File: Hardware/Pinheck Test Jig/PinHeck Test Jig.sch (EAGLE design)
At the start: 314 parts, among them U1 P8X32A-Q44, U10 BSO080P03NS3E G, U11 BSO080P03NS3E G, U12 MF-DSC-SOT233-MMBT3904, U13 MF-DSC-SOT233-MMBT3904, U14 CD74HC595M96, U15 CD74HC595M96, U16 CD74HC165M96, U17 CD74HC165M96, U18 CD74HC165M96, U19 CD74HC165M96, U2 CAT24C512WI-GT3, U20 CD74HC165M96, U21 CD74HC165M96, U22 CD74HC165M96, U23 CD74HC165M96, U24 CD74HC165M96, U26 CD74HC165M96, U27 CD74HC165M96, U28 CD74HC165M96, U29 CD74HC165M96, U3 FT230XS, U30 CD74HC165M96, U4 IP4234CZ6, U5 NCP1117DT33G, U6 NCP1117DT50G, U7 INA139NA/3K, U8 INA139NA/3K, U9 MAX11613EUA+, X1 ABMM-6.000MHZ-B2-T

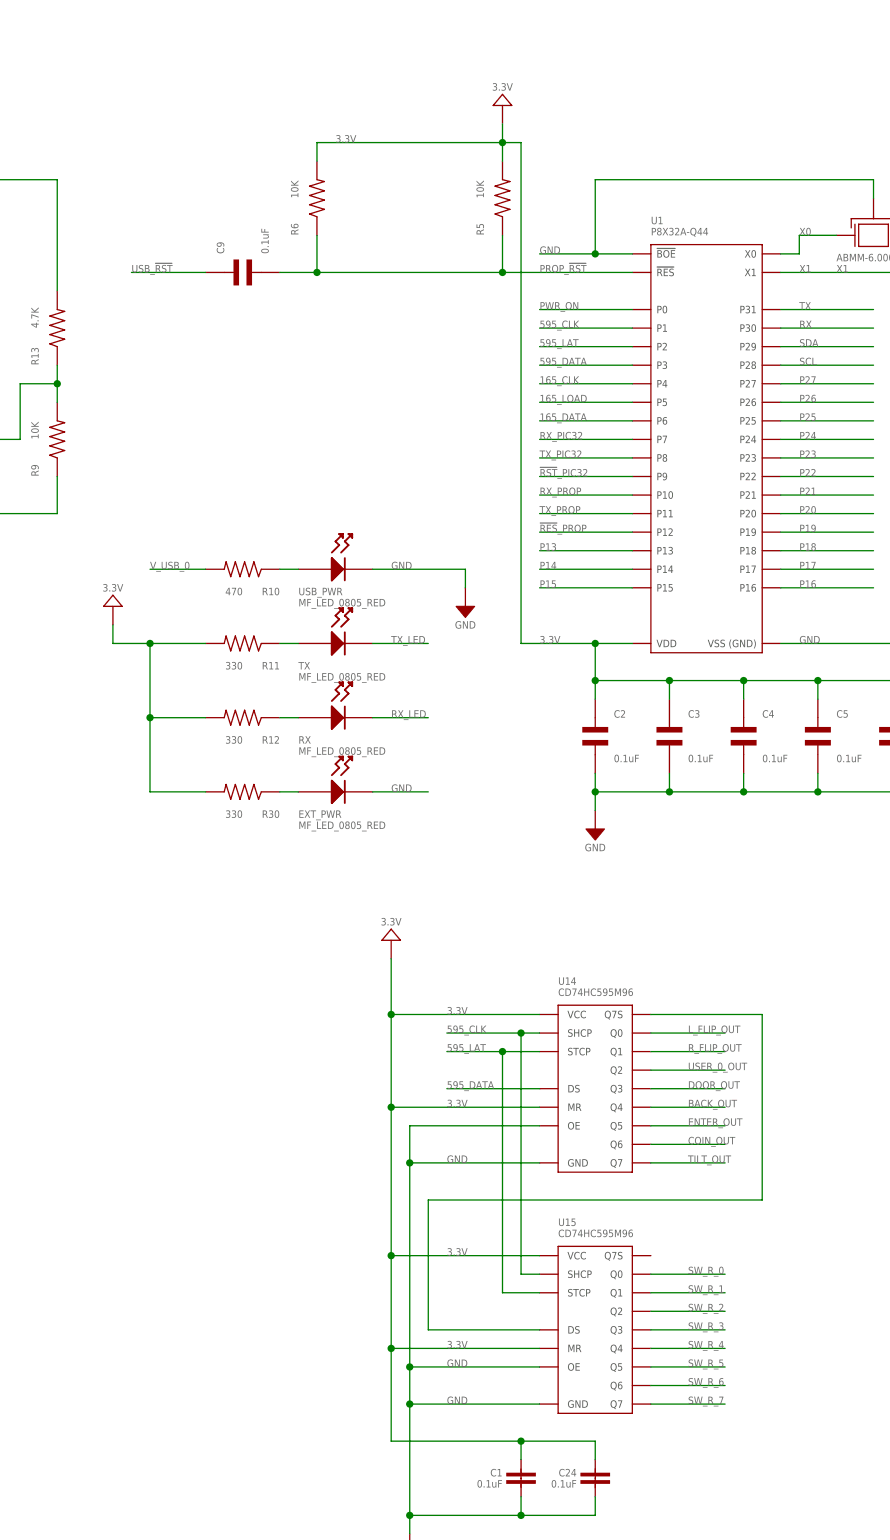
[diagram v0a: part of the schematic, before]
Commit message: Still routing!
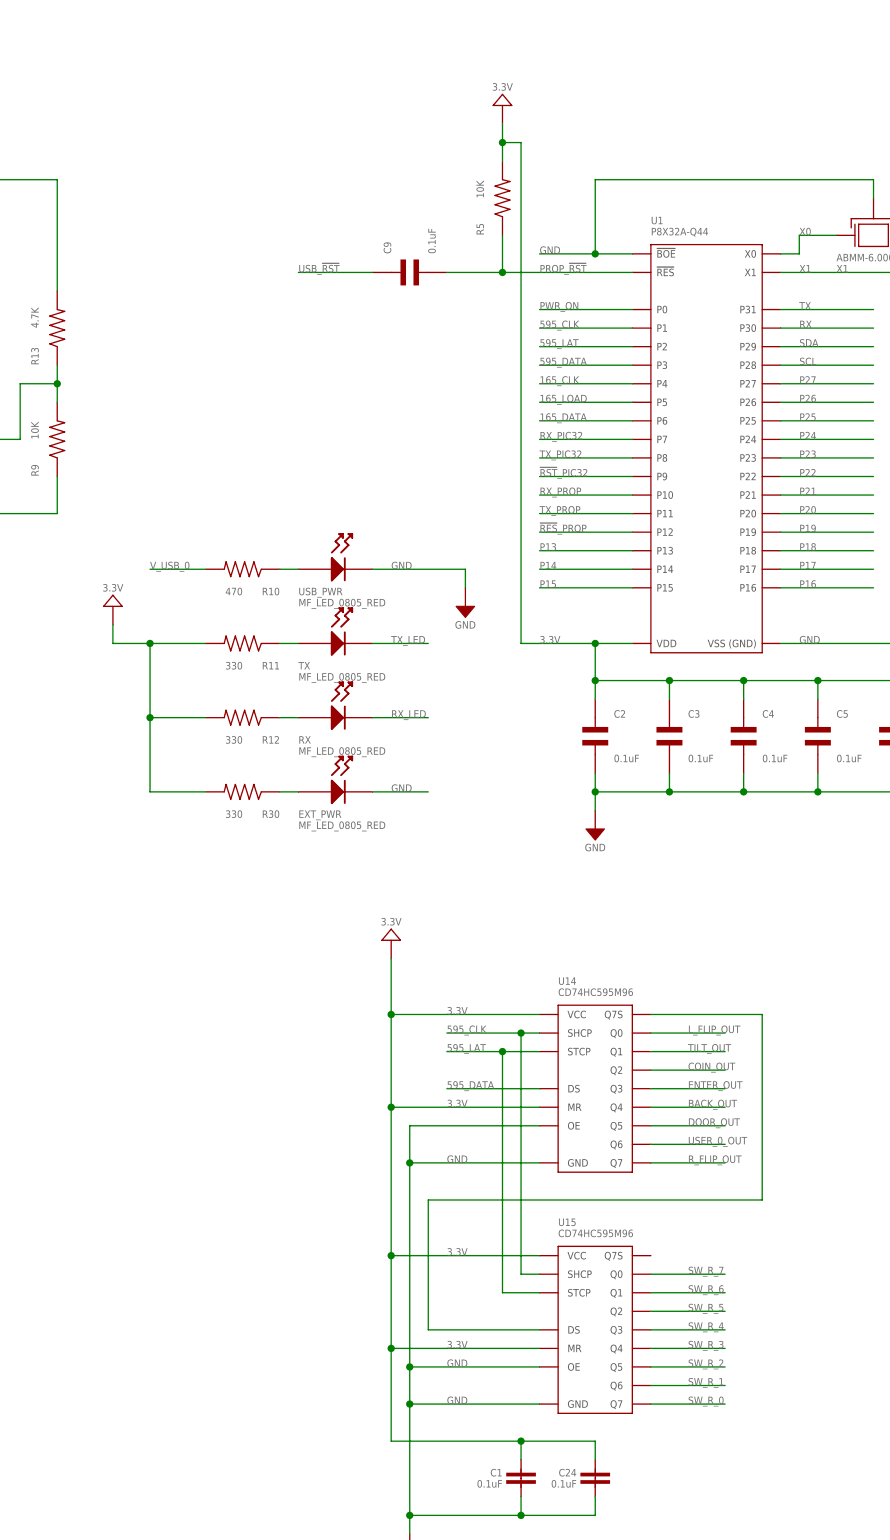
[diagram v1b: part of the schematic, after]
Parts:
- removed R6: 10K, MF_Passives:RESISTOR_0603
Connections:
- net 3.3V: no longer R6.P$2
- net COIN_OUT: now also U14.Q2; no longer U14.Q6
- net DOOR_OUT: now also U14.Q5; no longer U14.Q3
- net ENTER_OUT: now also U14.Q3; no longer U14.Q5
- net PROP_!RST: no longer R6.P$1
- net R_FLIP_OUT: now also U14.Q7; no longer U14.Q1
- net SW_R_0: now also U15.Q7; no longer U15.Q0
- net SW_R_1: now also U15.Q6; no longer U15.Q1
- net SW_R_2: now also U15.Q5; no longer U15.Q2
- net SW_R_3: now also U15.Q4; no longer U15.Q3
- net SW_R_4: now also U15.Q3; no longer U15.Q4
- net SW_R_5: now also U15.Q2; no longer U15.Q5
- net SW_R_6: now also U15.Q1; no longer U15.Q6
- net SW_R_7: now also U15.Q0; no longer U15.Q7
- net TILT_OUT: now also U14.Q1; no longer U14.Q7
- net USER_0_OUT: now also U14.Q6; no longer U14.Q2
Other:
- moved on the sheet: C9
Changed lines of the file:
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@@
 <?xml version="1.0" encoding="utf-8"?>
 <!DOCTYPE eagle SYSTEM "eagle.dtd">
-<eagle version="6.6.0">
+<eagle version="6.5.0">
 <drawing>
 <settings>
@@
 <part name="C6" library="MF_Passives" deviceset="CAPACITOR_NP" device="_0603" value="0.1uF"/>
 <part name="R5" library="MF_Passives" deviceset="RESISTOR" device="_0603" value="10K"/>
-<part name="R6" library="MF_Passives" deviceset="RESISTOR" device="_0603" value="10K"/>
 <part name="U3" library="MF_IC_Digital" deviceset="FT230X" device="S"/>
 <part name="U4" library="PP_Passives" deviceset="IP4234CZ6" device="" value="IP4234CZ6"/>
@@
 <instance part="C6" gate="G$1" x="190.5" y="172.72"/>
 <instance part="R5" gate="G$1" x="81.28" y="175.26" rot="R90"/>
-<instance part="R6" gate="G$1" x="55.88" y="175.26" rot="R90"/>
 <instance part="U3" gate="G$1" x="-17.78" y="165.1"/>
 <instance part="U4" gate="G$1" x="-91.44" y="152.4" rot="R90"/>
@@
 <instance part="J1" gate="G$1" x="-129.54" y="160.02"/>
 <instance part="L1" gate="G$1" x="-111.76" y="132.08"/>
-<instance part="C9" gate="G$1" x="45.72" y="165.1" rot="R90"/>
+<instance part="C9" gate="G$1" x="68.58" y="165.1" rot="R90"/>
 <instance part="C10" gate="G$1" x="-30.48" y="144.78"/>
 <instance part="C11" gate="G$1" x="-45.72" y="144.78"/>
@@
 <pinref part="R5" gate="G$1" pin="P$2"/>
 <wire x1="81.28" y1="180.34" x2="81.28" y2="182.88" width="0.1524" layer="91"/>
-<wire x1="81.28" y1="182.88" x2="55.88" y2="182.88" width="0.1524" layer="91"/>
-<pinref part="R6" gate="G$1" pin="P$2"/>
-<wire x1="55.88" y1="182.88" x2="55.88" y2="180.34" width="0.1524" layer="91"/>
-<label x="58.42" y="182.88" size="1.016" layer="95" font="vector"/>
 <pinref part="U$12" gate="G$1" pin="P$1"/>
 <wire x1="81.28" y1="182.88" x2="81.28" y2="185.42" width="0.1524" layer="91"/>
@@
 </segment>
 <segment>
-<pinref part="U15" gate="G$1" pin="Q6"/>
-<wire x1="111.76" y1="12.7" x2="101.6" y2="12.7" width="0.1524" layer="91"/>
-<label x="106.68" y="12.7" size="1.016" layer="95" font="vector"/>
+<pinref part="U15" gate="G$1" pin="Q1"/>
+<wire x1="101.6" y1="25.4" x2="111.76" y2="25.4" width="0.1524" layer="91"/>
+<label x="106.68" y="25.4" size="1.016" layer="95" font="vector"/>
 </segment>
 </net>
@@
 </segment>
 <segment>
-<pinref part="U15" gate="G$1" pin="Q5"/>
-<wire x1="101.6" y1="15.24" x2="111.76" y2="15.24" width="0.1524" layer="91"/>
-<label x="106.68" y="15.24" size="1.016" layer="95" font="vector"/>
+<pinref part="U15" gate="G$1" pin="Q2"/>
+<wire x1="111.76" y1="22.86" x2="101.6" y2="22.86" width="0.1524" layer="91"/>
+<label x="106.68" y="22.86" size="1.016" layer="95" font="vector"/>
 </segment>
 </net>
@@
 </segment>
 <segment>
-<pinref part="U15" gate="G$1" pin="Q4"/>
-<wire x1="111.76" y1="17.78" x2="101.6" y2="17.78" width="0.1524" layer="91"/>
-<label x="106.68" y="17.78" size="1.016" layer="95" font="vector"/>
+<pinref part="U15" gate="G$1" pin="Q3"/>
+<wire x1="101.6" y1="20.32" x2="111.76" y2="20.32" width="0.1524" layer="91"/>
+<label x="106.68" y="20.32" size="1.016" layer="95" font="vector"/>
 </segment>
 </net>
@@
 </segment>
 <segment>
-<pinref part="U15" gate="G$1" pin="Q3"/>
-<wire x1="101.6" y1="20.32" x2="111.76" y2="20.32" width="0.1524" layer="91"/>
-<label x="106.68" y="20.32" size="1.016" layer="95" font="vector"/>
+<pinref part="U15" gate="G$1" pin="Q4"/>
+<wire x1="111.76" y1="17.78" x2="101.6" y2="17.78" width="0.1524" layer="91"/>
+<label x="106.68" y="17.78" size="1.016" layer="95" font="vector"/>
 </segment>
 </net>
@@
 </segment>
 <segment>
-<pinref part="U15" gate="G$1" pin="Q1"/>
-<wire x1="101.6" y1="25.4" x2="111.76" y2="25.4" width="0.1524" layer="91"/>
-<label x="106.68" y="25.4" size="1.016" layer="95" font="vector"/>
+<pinref part="U15" gate="G$1" pin="Q6"/>
+<wire x1="111.76" y1="12.7" x2="101.6" y2="12.7" width="0.1524" layer="91"/>
+<label x="106.68" y="12.7" size="1.016" layer="95" font="vector"/>
 </segment>
 </net>
@@
 </segment>
 <segment>
-<pinref part="U15" gate="G$1" pin="Q0"/>
-<wire x1="101.6" y1="27.94" x2="111.76" y2="27.94" width="0.1524" layer="91"/>
-<label x="106.68" y="27.94" size="1.016" layer="95" font="vector"/>
+<pinref part="U15" gate="G$1" pin="Q7"/>
+<wire x1="101.6" y1="10.16" x2="111.76" y2="10.16" width="0.1524" layer="91"/>
+<label x="106.68" y="10.16" size="1.016" layer="95" font="vector"/>
 </segment>
 </net>
@@
 </segment>
 <segment>
-<pinref part="U15" gate="G$1" pin="Q7"/>
-<wire x1="101.6" y1="10.16" x2="111.76" y2="10.16" width="0.1524" layer="91"/>
-<label x="106.68" y="10.16" size="1.016" layer="95" font="vector"/>
+<pinref part="U15" gate="G$1" pin="Q0"/>
+<wire x1="101.6" y1="27.94" x2="111.76" y2="27.94" width="0.1524" layer="91"/>
+<label x="106.68" y="27.94" size="1.016" layer="95" font="vector"/>
 </segment>
 </net>
@@
 </segment>
 <segment>
-<pinref part="U15" gate="G$1" pin="Q2"/>
-<wire x1="111.76" y1="22.86" x2="101.6" y2="22.86" width="0.1524" layer="91"/>
-<label x="106.68" y="22.86" size="1.016" layer="95" font="vector"/>
+<pinref part="U15" gate="G$1" pin="Q5"/>
+<wire x1="101.6" y1="15.24" x2="111.76" y2="15.24" width="0.1524" layer="91"/>
+<label x="106.68" y="15.24" size="1.016" layer="95" font="vector"/>
 </segment>
 </net>
@@
 </segment>
 <segment>
-<pinref part="U14" gate="G$1" pin="Q7"/>
-<wire x1="101.6" y1="43.18" x2="111.76" y2="43.18" width="0.1524" layer="91"/>
-<label x="106.68" y="43.18" size="1.016" layer="95" font="vector"/>
+<pinref part="U14" gate="G$1" pin="Q1"/>
+<wire x1="101.6" y1="58.42" x2="111.76" y2="58.42" width="0.1524" layer="91"/>
+<label x="106.68" y="58.42" size="1.016" layer="95" font="vector"/>
 </segment>
 </net>
@@
 </segment>
 <segment>
-<pinref part="U14" gate="G$1" pin="Q6"/>
-<wire x1="111.76" y1="45.72" x2="101.6" y2="45.72" width="0.1524" layer="91"/>
-<label x="106.68" y="45.72" size="1.016" layer="95" font="vector"/>
+<pinref part="U14" gate="G$1" pin="Q2"/>
+<wire x1="111.76" y1="55.88" x2="101.6" y2="55.88" width="0.1524" layer="91"/>
+<label x="106.68" y="55.88" size="1.016" layer="95" font="vector"/>
 </segment>
 </net>
@@
 </segment>
 <segment>
-<pinref part="U14" gate="G$1" pin="Q5"/>
-<wire x1="101.6" y1="48.26" x2="111.76" y2="48.26" width="0.1524" layer="91"/>
-<label x="106.68" y="48.26" size="1.016" layer="95" font="vector"/>
+<pinref part="U14" gate="G$1" pin="Q3"/>
+<wire x1="101.6" y1="53.34" x2="111.76" y2="53.34" width="0.1524" layer="91"/>
+<label x="106.68" y="53.34" size="1.016" layer="95" font="vector"/>
 </segment>
 </net>
@@
 </segment>
 <segment>
-<pinref part="U14" gate="G$1" pin="Q3"/>
-<wire x1="101.6" y1="53.34" x2="111.76" y2="53.34" width="0.1524" layer="91"/>
-<label x="106.68" y="53.34" size="1.016" layer="95" font="vector"/>
+<pinref part="U14" gate="G$1" pin="Q5"/>
+<wire x1="101.6" y1="48.26" x2="111.76" y2="48.26" width="0.1524" layer="91"/>
+<label x="106.68" y="48.26" size="1.016" layer="95" font="vector"/>
 </segment>
 </net>
@@
 </segment>
 <segment>
-<pinref part="U14" gate="G$1" pin="Q2"/>
-<wire x1="111.76" y1="55.88" x2="101.6" y2="55.88" width="0.1524" layer="91"/>
-<label x="106.68" y="55.88" size="1.016" layer="95" font="vector"/>
+<pinref part="U14" gate="G$1" pin="Q6"/>
+<wire x1="111.76" y1="45.72" x2="101.6" y2="45.72" width="0.1524" layer="91"/>
+<label x="106.68" y="45.72" size="1.016" layer="95" font="vector"/>
 </segment>
 </net>
@@
 </segment>
 <segment>
-<pinref part="U14" gate="G$1" pin="Q1"/>
-<wire x1="101.6" y1="58.42" x2="111.76" y2="58.42" width="0.1524" layer="91"/>
-<label x="106.68" y="58.42" size="1.016" layer="95" font="vector"/>
+<pinref part="U14" gate="G$1" pin="Q7"/>
+<wire x1="101.6" y1="43.18" x2="111.76" y2="43.18" width="0.1524" layer="91"/>
+<label x="106.68" y="43.18" size="1.016" layer="95" font="vector"/>
 </segment>
 </net>
@@
 <junction x="81.28" y="165.1"/>
 <pinref part="C9" gate="G$1" pin="P$2"/>
-<wire x1="50.8" y1="165.1" x2="55.88" y2="165.1" width="0.1524" layer="91"/>
-<pinref part="R6" gate="G$1" pin="P$1"/>
-<wire x1="55.88" y1="165.1" x2="81.28" y2="165.1" width="0.1524" layer="91"/>
-<wire x1="55.88" y1="170.18" x2="55.88" y2="165.1" width="0.1524" layer="91"/>
-<junction x="55.88" y="165.1"/>
+<wire x1="73.66" y1="165.1" x2="81.28" y2="165.1" width="0.1524" layer="91"/>
 </segment>
 </net>
@@
 <segment>
 <pinref part="C9" gate="G$1" pin="P$1"/>
-<wire x1="30.48" y1="165.1" x2="40.64" y2="165.1" width="0.1524" layer="91"/>
-<label x="30.48" y="165.1" size="1.016" layer="95" font="vector"/>
+<wire x1="53.34" y1="165.1" x2="63.5" y2="165.1" width="0.1524" layer="91"/>
+<label x="53.34" y="165.1" size="1.016" layer="95" font="vector"/>
 </segment>
 </net>
